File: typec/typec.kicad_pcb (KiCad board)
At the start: 2 copper layers, 76 parts, among them U1 TPD6E05U06-USON, U2 TPD4E05U06-USON, U3 TPS62081-WSON, U4 TPD4E05U06-USON, U5 TPS74801-VSON, U6 TUSB212-X2QFN, U7 USB_HUB, Y1 24 MHz

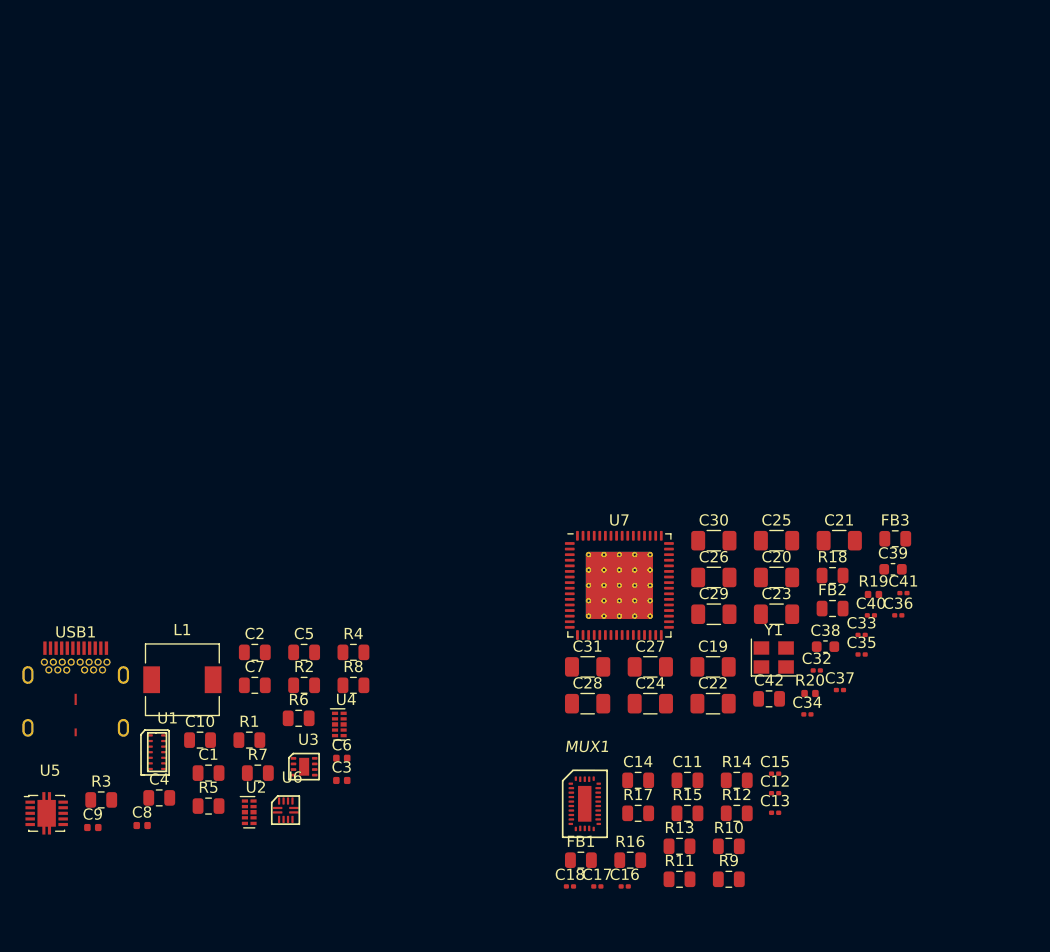
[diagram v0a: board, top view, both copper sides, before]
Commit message: Last minute changes
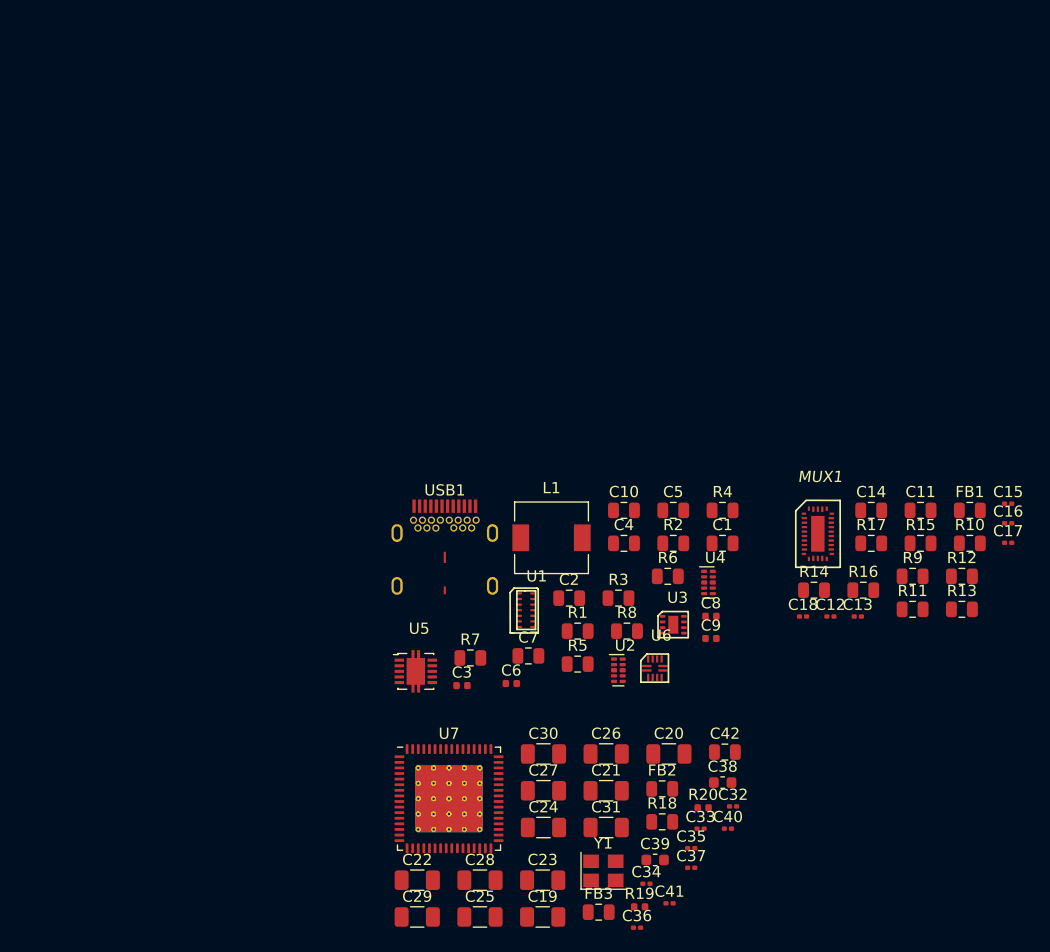
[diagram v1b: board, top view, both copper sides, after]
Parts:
- moved C9 57.8 mm to (154.3, 87.4)
- moved C8 54.2 mm to (154.3, 85.4)
- moved C1 50.4 mm to (155.3, 78.9)
- moved R3 49.7 mm to (146.0, 83.8)
- moved C17 47.9 mm to (180.9, 78.8)
- moved C4 47.4 mm to (146.5, 78.9)
- moved C16 47.2 mm to (180.9, 77.1)
- moved FB1 46.8 mm to (177.5, 75.9)
- moved C10 43.1 mm to (146.5, 75.9)
- moved C25 42.9 mm to (133.6, 112.3)
- moved FB3 42.7 mm to (144.3, 111.8)
- moved C29 37.9 mm to (128.0, 112.3)
- moved C36 36.4 mm to (147.7, 113.2)
- moved L1 35.4 mm to (140.0, 78.4)
- moved C5 35.4 mm to (150.9, 75.9)
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
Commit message: updated
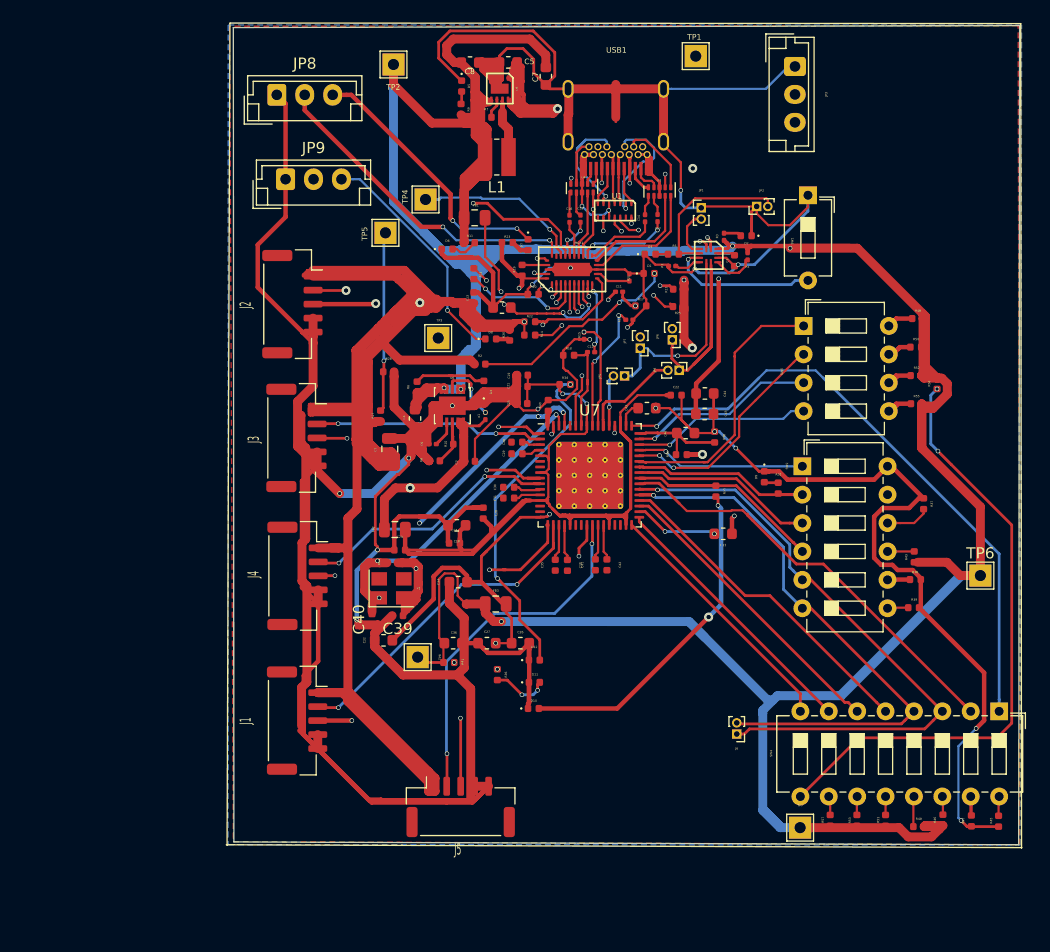
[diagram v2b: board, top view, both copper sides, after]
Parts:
- removed C37: 0.1uF/10v, Capacitor_SMD:C_0201_0603Metric
- removed C9: 0.1uF/10v, Capacitor_SMD:C_0402_1005Metric
- added C43: 1uF/10v, Capacitor_SMD:C_0603_1608Metric, F.Cu at (148.6, 66.8)
- added C44: 1uf/10v, Capacitor_SMD:C_0603_1608Metric, F.Cu at (153.8, 65.4)
- added C45: 1uf/10v, Capacitor_SMD:C_0603_1608Metric, F.Cu at (153.7, 67.3)
- added C46: 10 uF/10v, Capacitor_SMD:C_0603_1608Metric, F.Cu at (152.0, 69.0)
- added D1: LED, LED_SMD:LED_0402_1005Metric, F.Cu at (148.8, 54.7)
- added D10: LED, LED_SMD:LED_0402_1005Metric, F.Cu at (138.4, 93.6)
- added D11: LED, LED_SMD:LED_0402_1005Metric, F.Cu at (138.5, 91.3)
- added D12: LED, LED_SMD:LED_0402_1005Metric, F.Cu at (138.5, 89.3)
- added D2: LED, LED_SMD:LED_0402_1005Metric, F.Cu at (157.5, 51.3)
- added D3: LED, LED_SMD:LED_0402_1005Metric, F.Cu at (148.9, 53.0)
- added D4: LED, LED_SMD:LED_0402_1005Metric, F.Cu at (134.0, 64.8)
- added D5: LED, LED_SMD:LED_0402_1005Metric, F.Cu at (132.0, 38.0)
- added D6: LED, LED_SMD:LED_0402_1005Metric, F.Cu at (130.7, 52.5)
- added D7: LED, LED_SMD:LED_0402_1005Metric, F.Cu at (137.9, 52.1)
- added D8: LED, LED_SMD:LED_0402_1005Metric, F.Cu at (134.6, 60.6)
- added D9: LED, LED_SMD:LED_0402_1005Metric, F.Cu at (159.1, 72.9)
- added J1: Conn_01x05_Female, Connector_JST:JST_GH_SM05B-GHS-TB_1x05-1MP_P1.25mm_Horizontal, F.Cu at (117.3, 94.7)
- added J2: Conn_01x05_Female, Connector_JST:JST_GH_SM05B-GHS-TB_1x05-1MP_P1.25mm_Horizontal, F.Cu at (116.9, 57.5)
- added J3: Conn_01x05_Female, Connector_JST:JST_GH_SM05B-GHS-TB_1x05-1MP_P1.25mm_Horizontal, F.Cu at (117.2, 69.4)
- added J4: Conn_01x05_Female, Connector_JST:JST_GH_SM05B-GHS-TB_1x05-1MP_P1.25mm_Horizontal, F.Cu at (117.3, 81.8)
- added J5: Conn_01x05_Female, Connector_JST:JST_GH_SM05B-GHS-TB_1x05-1MP_P1.25mm_Horizontal, F.Cu at (131.9, 102.4)
- added J6: Conn_01x02_Female, Connector_PinHeader_1.00mm:PinHeader_1x02_P1.00mm_Vertical, F.Cu at (156.6, 95.9)
- added JP1: Jumper_NO_Small, Connector_PinHeader_1.00mm:PinHeader_1x02_P1.00mm_Vertical, F.Cu at (153.4, 48.8)
- added JP2: Jumper_NO_Small, Connector_PinHeader_1.00mm:PinHeader_1x02_P1.00mm_Vertical, F.Cu at (158.4, 48.7)
- added JP3: Jumper_3_Open, Connector_JST:JST_EH_B3B-EH-A_1x03_P2.50mm_Vertical, F.Cu at (161.8, 36.2)
- added JP4: Jumper_2_Open, Connector_PinHeader_1.00mm:PinHeader_1x02_P1.00mm_Vertical, F.Cu at (151.5, 63.4)
- added JP5: Jumper_2_Open, Connector_PinHeader_1.00mm:PinHeader_1x02_P1.00mm_Vertical, F.Cu at (146.6, 63.9)
- added JP6: Jumper_2_Open, Connector_PinHeader_1.00mm:PinHeader_1x02_P1.00mm_Vertical, F.Cu at (150.9, 60.7)
- added JP7: Jumper_2_Open, Connector_PinHeader_1.00mm:PinHeader_1x02_P1.00mm_Vertical, F.Cu at (148.0, 61.4)
- added JP8: Jumper_3_Open, Connector_JST:JST_EH_B3B-EH-A_1x03_P2.50mm_Vertical, F.Cu at (115.5, 38.7)
- added JP9: Jumper_3_Open, Connector_JST:JST_EH_B3B-EH-A_1x03_P2.50mm_Vertical, F.Cu at (116.3, 46.3)
- added R21: 0 E, Resistor_SMD:R_0201_0603Metric, F.Cu at (147.0, 55.1)
- added R22: 200 K, Resistor_SMD:R_0402_1005Metric, F.Cu at (138.1, 59.0)
- added R23: 500 E, Resistor_SMD:R_0402_1005Metric, F.Cu at (136.1, 51.9)
- added R25: 200 K, Resistor_SMD:R_0402_1005Metric, F.Cu at (151.4, 57.7)
- added R26: 500 E, Resistor_SMD:R_0402_1005Metric, F.Cu at (136.3, 60.2)
- added R27: NC / 10 K, Resistor_SMD:R_0402_1005Metric, F.Cu at (124.8, 67.5)
- added R28: NC/ 10 K, Resistor_SMD:R_0402_1005Metric, F.Cu at (125.5, 63.5)
- added R31: 330 E, Resistor_SMD:R_0402_1005Metric, F.Cu at (160.3, 73.9)
- added R34: 330 E, Resistor_SMD:R_0402_1005Metric, F.Cu at (141.2, 64.6)
- added R35: 330 E, Resistor_SMD:R_0402_1005Metric, F.Cu at (154.7, 74.2)
- added R36: 330 E, Resistor_SMD:R_0402_1005Metric, F.Cu at (135.2, 90.6)
- added R37: 1 K, Resistor_SMD:R_0402_1005Metric, F.Cu at (173.3, 75.3)
- added R38: 1 K, Resistor_SMD:R_0402_1005Metric, F.Cu at (172.6, 82.1)
- added R39: 1 K, Resistor_SMD:R_0402_1005Metric, F.Cu at (172.4, 84.6)
- added R40: 9.53 K, Resistor_SMD:R_0402_1005Metric, F.Cu at (139.8, 66.5)
- added R41: 1 K, Resistor_SMD:R_0402_1005Metric, F.Cu at (130.9, 89.5)
- added R43: 1 K, Resistor_SMD:R_0402_1005Metric, F.Cu at (172.5, 80.1)
- added R44: 1 M, Resistor_SMD:R_0402_1005Metric, F.Cu at (125.8, 80.6)
- added R45: 1 K, Resistor_SMD:R_0402_1005Metric, F.Cu at (180.0, 103.7)
- added R46: 1 K, Resistor_SMD:R_0402_1005Metric, F.Cu at (175.1, 103.6)
- added R47: 1 K, Resistor_SMD:R_0402_1005Metric, F.Cu at (177.6, 103.7)
- added R48: 10 K, Resistor_SMD:R_0402_1005Metric, F.Cu at (172.8, 58.7)
- added R49: 1 K, Resistor_SMD:R_0402_1005Metric, F.Cu at (172.9, 104.2)
- added R50: 10 K, Resistor_SMD:R_0402_1005Metric, F.Cu at (172.6, 61.3)
- added R51: 4.7 K, Resistor_SMD:R_0402_1005Metric, F.Cu at (169.9, 103.6)
- added R52: 10 K, Resistor_SMD:R_0402_1005Metric, F.Cu at (172.7, 63.8)
- added R53: 4.7 K, Resistor_SMD:R_0402_1005Metric, F.Cu at (167.4, 103.6)
- added R54: 90.9 K, Resistor_SMD:R_0402_1005Metric, F.Cu at (151.7, 70.9)
- added R55: 10 K, Resistor_SMD:R_0402_1005Metric, F.Cu at (172.7, 66.4)
- added R56: 10 K, Resistor_SMD:R_0402_1005Metric, F.Cu at (154.6, 69.3)
- added R57: 4.7 K, Resistor_SMD:R_0402_1005Metric, F.Cu at (165.0, 103.6)
- added R58: 4.7 K, Resistor_SMD:R_0402_1005Metric, F.Cu at (174.5, 64.6)
- added SW1: SW_Push_Dual_x2, Button_Switch_THT:SW_DIP_SPSTx01_Slide_6.7x4.1mm_W7.62mm_P2.54mm_LowProfile, F.Cu at (163.0, 47.7)
- added SW2: SW_DIP_x06, Button_Switch_THT:SW_DIP_SPSTx06_Slide_6.7x16.8mm_W7.62mm_P2.54mm_LowProfile, F.Cu at (162.5, 72.0)
- added SW4: SW_DIP_x08, Button_Switch_THT:SW_DIP_SPSTx08_Slide_6.7x21.88mm_W7.62mm_P2.54mm_LowProfile, F.Cu at (180.1, 93.9)
- added SW5: SW_DIP_x04, Button_Switch_THT:SW_DIP_SPSTx04_Slide_6.7x11.72mm_W7.62mm_P2.54mm_LowProfile, F.Cu at (162.6, 59.4)
- added TP1: TestPoint, TestPoint:TestPoint_THTPad_2.0x2.0mm_Drill1.0mm, F.Cu at (152.9, 35.3)
- added TP2: TestPoint, TestPoint:TestPoint_THTPad_2.0x2.0mm_Drill1.0mm, F.Cu at (125.9, 36.0)
- added TP3: TestPoint, TestPoint:TestPoint_THTPad_2.0x2.0mm_Drill1.0mm, F.Cu at (129.9, 60.5)
- added TP4: TestPoint, TestPoint:TestPoint_THTPad_2.0x2.0mm_Drill1.0mm, F.Cu at (128.8, 48.1)
- added TP5: TestPoint, TestPoint:TestPoint_THTPad_2.0x2.0mm_Drill1.0mm, F.Cu at (125.2, 51.1)
- added TP6: TestPoint, TestPoint:TestPoint_THTPad_2.0x2.0mm_Drill1.0mm, F.Cu at (178.4, 81.7)
- added TP7: TestPoint, TestPoint:TestPoint_THTPad_2.0x2.0mm_Drill1.0mm, F.Cu at (162.3, 104.3)
- added TP8: TestPoint, TestPoint:TestPoint_THTPad_2.0x2.0mm_Drill1.0mm, F.Cu at (128.1, 89.0)
- added e1: 105 K, Resistor_SMD:R_0201_0603Metric, F.Cu at (134.1, 67.5)
- C10: value 10uf/10v -> 0.1uf/10v; footprint Capacitor_SMD:C_0805_2012Metric -> Capacitor_SMD:C_0603_1608Metric
- C11: value 0.1uf/10v -> 0.47uf/10v; footprint Capacitor_SMD:C_0805_2012Metric -> Capacitor_SMD:C_0201_0603Metric
- C13: value 0.47uf/10v -> 4.7uf/10v; footprint Capacitor_SMD:C_0201_0603Metric -> Capacitor_SMD:C_0402_1005Metric
- C14: value 47uf/10v -> 0.4uf/10v; footprint Capacitor_SMD:C_0805_2012Metric -> Capacitor_SMD:C_0201_0603Metric
- C15: value 0.4uf/10v -> 0.47uf/10v
- C16: value 0.47uf/10v -> 0.4uf/10v
- C18: value 0.4uf/10v -> 10uF/10v; footprint Capacitor_SMD:C_0201_0603Metric -> Capacitor_SMD:C_0603_1608Metric
- C19, C20, C21, C22, C23, C24, C25, C28, C29, C30: footprint Capacitor_SMD:C_1206_3216Metric -> Capacitor_SMD:C_0402_1005Metric
- C2: value 10uf/10v -> 0.1uF/10v; footprint Capacitor_SMD:C_0805_2012Metric -> Capacitor_SMD:C_0402_1005Metric
- C26: value 10uF/10v -> 0.1uF/10v; footprint Capacitor_SMD:C_1206_3216Metric -> Capacitor_SMD:C_0603_1608Metric
- C27: footprint Capacitor_SMD:C_1206_3216Metric -> Capacitor_SMD:C_0603_1608Metric
- C3: value 1uf/10v -> 10uf/10v
- C31: value 10uF/10v -> 0.1uF/10v; footprint Capacitor_SMD:C_1206_3216Metric -> Capacitor_SMD:C_0402_1005Metric
- C32, C33: footprint Capacitor_SMD:C_0201_0603Metric -> Capacitor_SMD:C_0603_1608Metric
- C34: value 0.1uF/10v -> 10uF/10v; footprint Capacitor_SMD:C_0201_0603Metric -> Capacitor_SMD:C_0603_1608Metric
- C35, C41: footprint Capacitor_SMD:C_0201_0603Metric -> Capacitor_SMD:C_0402_1005Metric
- C36: value 0.1uF/10v -> 1uf/10v; footprint Capacitor_SMD:C_0201_0603Metric -> Capacitor_SMD:C_0603_1608Metric
- C38: value 18pF/10v -> 0.1uF/10v; footprint Capacitor_SMD:C_0603_1608Metric -> Capacitor_SMD:C_0402_1005Metric
- C39: footprint Capacitor_SMD:C_0603_1608Metric -> Capacitor_SMD:C_0402_1005Metric
- C4: value 10 uF/10V -> 1uf/10v; footprint Capacitor_SMD:C_0805_2012Metric -> Capacitor_SMD:C_0603_1608Metric
- C40: value 0.1uF/10v -> 18pF/10v; footprint Capacitor_SMD:C_0201_0603Metric -> Capacitor_SMD:C_0402_1005Metric
- C42: value 1uF/10v -> 0.1uF/10v; footprint Capacitor_SMD:C_0805_2012Metric -> Capacitor_SMD:C_0402_1005Metric
- C5: value 22uf/6.3v -> 10 uF/10V; footprint Capacitor_SMD:C_0805_2012Metric -> Capacitor_SMD:C_0603_1608Metric
- C6: value 560pf/10v -> 590pf/10v; footprint Capacitor_SMD:C_0402_1005Metric -> Capacitor_SMD:C_0201_0603Metric
- C7: value 10uf/10v -> 22uf/6.3v; footprint Capacitor_SMD:C_0805_2012Metric -> Capacitor_SMD:C_0603_1608Metric
- C8: value 0.1uF/10v -> 10uf/10v; footprint Capacitor_SMD:C_0402_1005Metric -> Capacitor_SMD:C_0603_1608Metric
- L1: footprint Inductor_SMD:L_6.3x6.3_H3 -> Inductor_SMD:L_Wuerth_MAPI-3015
- R1: value 105 K -> 1.6K; footprint Resistor_SMD:R_0805_2012Metric -> Resistor_SMD:R_0201_0603Metric
- R10: value 10 K -> 1.9K; footprint Resistor_SMD:R_0805_2012Metric -> Resistor_SMD:R_0402_1005Metric
- R11: value 900 K -> 330 E; footprint Resistor_SMD:R_0805_2012Metric -> Resistor_SMD:R_0402_1005Metric
- R12, R15: footprint Resistor_SMD:R_0805_2012Metric -> Resistor_SMD:R_0201_0603Metric
- R13: value 4.7K -> 10 K; footprint Resistor_SMD:R_0805_2012Metric -> Resistor_SMD:R_0402_1005Metric
- R14: value 100K -> 900 K; footprint Resistor_SMD:R_0805_2012Metric -> Resistor_SMD:R_0402_1005Metric
- R16: value 0 E -> 4.7K; footprint Resistor_SMD:R_0805_2012Metric -> Resistor_SMD:R_0402_1005Metric
- R17: value 0 E -> 100K; footprint Resistor_SMD:R_0805_2012Metric -> Resistor_SMD:R_0402_1005Metric
- R18: value 1 M -> 100K; footprint Resistor_SMD:R_0805_2012Metric -> Resistor_SMD:R_0402_1005Metric
- R19: value 4.7K -> 200 K
- R2: value 178K -> 330 E; footprint Resistor_SMD:R_0805_2012Metric -> Resistor_SMD:R_0402_1005Metric
- R20: value 4.7K -> 0 E
- R3: value 5 K -> 330 E; footprint Resistor_SMD:R_0805_2012Metric -> Resistor_SMD:R_0201_0603Metric
- R4: value 1.9K -> 43K; footprint Resistor_SMD:R_0805_2012Metric -> Resistor_SMD:R_0201_0603Metric
- R5: value 1.6K -> 100 E; footprint Resistor_SMD:R_0805_2012Metric -> Resistor_SMD:R_0402_1005Metric
- R6: value 43K -> 330 E; footprint Resistor_SMD:R_0805_2012Metric -> Resistor_SMD:R_0402_1005Metric
- R7: value 0 E -> 178K; footprint Resistor_SMD:R_0805_2012Metric -> Resistor_SMD:R_0402_1005Metric
- R8: value 0 E -> 5 K; footprint Resistor_SMD:R_0805_2012Metric -> Resistor_SMD:R_0402_1005Metric
- R9: value 100K -> 330 E; footprint Resistor_SMD:R_0805_2012Metric -> Resistor_SMD:R_0402_1005Metric
- U2: value TPD4E05U06-USON -> TUSB212-X2QFN; footprint TPD4E05U06-USON:TPD4E05U06-USON -> TUSB212-X2QFN:TUSB212-X2QFN
- U3: value TPS62081-WSON -> TPD4E05U06-USON; footprint TPS62081-WSON:TPS62081-WSON -> TPD4E05U06-USON:TPD4E05U06-USON
- U5: value TPS74801-VSON -> TPS62082-WSON; footprint TPS74801-VSON:TPS74801-VSON -> TPS62081-WSON:TPS62082-WSON
- U6: value TUSB212-X2QFN -> TPS74801-VSON; footprint TUSB212-X2QFN:TUSB212-X2QFN -> TPS74801-VSON:TPS74801-VSON
- moved R9 58.1 mm to (132.0, 40.0), turned to 90 degrees
- moved R19 57.9 mm to (137.4, 54.4), turned to 270 degrees
- moved C8 54.0 mm to (132.8, 35.8)
- moved USB1 53.6 mm to (145.8, 34.7), turned to 180 degrees
- moved U5 52.8 mm to (135.0, 37.9), turned to 270 degrees
- moved C7 51.9 mm to (139.5, 37.1), turned to 270 degrees
- moved R11 51.5 mm to (132.7, 52.0)
- moved FB1 51.4 mm to (133.2, 49.7)
- moved C22 49.2 mm to (151.2, 65.6), turned to 180 degrees
- moved C19 48.5 mm to (137.4, 63.8)
- moved R20 48.4 mm to (138.4, 56.6)
- moved R7 48.4 mm to (134.2, 40.7), turned to 180 degrees
- moved C16 47.8 mm to (141.7, 49.8), turned to 90 degrees
- moved R10 46.6 mm to (131.7, 70.0), turned to 180 degrees
- moved C25 46.1 mm to (137.4, 66.3)
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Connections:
- C1 pad 1: VOUT(1.1V) -> VBUS
- C1 pad 2: USB3_RX0N -> GND
- C10 pad 1: VBUS -> Net-(C10-Pad1)
- C10 pad 2: USB3_RX0N -> GND
- C12 pad 2: USB3_RX0N -> USB3_RX0P
- C13 pad 1: Net-(C13-Pad1) -> GND
- C13 pad 2: USB3_RX0N -> VBUS
- C14 pad 1: USB3_RX0N -> CTX1N0
- C14 pad 2: VBUS -> Net-(C14-Pad2)
- C15 pad 1: CTX1N -> Net-(C15-Pad1)
- C15 pad 2: Net-(C15-Pad2) -> CTX2P0
- C16 pad 2: CTX2P -> CTX2N0
- C17 pad 2: CTX2N -> CTX1P0
- C18 pad 2: CTX1P -> GND
- C19 pad 1: USB3_RX0N -> GND
- C19 pad 2: Net-(C19-Pad2) -> Net-(C18-Pad1)
- C2 pad 1: VBUS -> Net-(C2-Pad1)
- C2 pad 2: USB3_RX0N -> GND
- C20 pad 1: USB3_RX0N -> GND
- C20 pad 2: Net-(C19-Pad2) -> Net-(C18-Pad1)
- C21 pad 1: USB3_RX0N -> GND
- C21 pad 2: Net-(C19-Pad2) -> Net-(C18-Pad1)
- C22 pad 1: USB3_RX0N -> GND
- C22 pad 2: Net-(C19-Pad2) -> Net-(C18-Pad1)
- C23 pad 1: USB3_RX0N -> GND
- C23 pad 2: Net-(C19-Pad2) -> Net-(C18-Pad1)
- C24 pad 1: USB3_RX0N -> GND
- C24 pad 2: Net-(C19-Pad2) -> Net-(C18-Pad1)
- C25 pad 1: USB3_RX0N -> GND
- C25 pad 2: Net-(C19-Pad2) -> Net-(C18-Pad1)
- C26 pad 1: Net-(C19-Pad2) -> GND
- C26 pad 2: USB3_RX0N -> Net-(C26-Pad2)
- C27 pad 1: USB3_RX0N -> GND
- C27 pad 2: Net-(C27-Pad2) -> Net-(C26-Pad2)
- C28 pad 1: USB3_RX0N -> (no net)
- C28 pad 2: Net-(C27-Pad2) -> Net-(C28-Pad2)
- C29 pad 1: USB3_RX0N -> Net-(C29-Pad1)
- C29 pad 2: Net-(C27-Pad2) -> (no net)
- C3 pad 1: Net-(C3-Pad1) -> VOUT(1.1V)
- C3 pad 2: USB3_RX0N -> GND
- C30 pad 1: USB3_RX0N -> (no net)
- C30 pad 2: Net-(C27-Pad2) -> Net-(C30-Pad2)
- C31 pad 1: Net-(C27-Pad2) -> Net-(C31-Pad1)
- C31 pad 2: USB3_RX0N -> (no net)
- C32 pad 1: Tx1+ -> GND
- C32 pad 2: Net-(C32-Pad2) -> Net-(C26-Pad2)
- C33 pad 1: Net-(C33-Pad1) -> GND
- C33 pad 2: Tx1- -> Net-(C26-Pad2)
- C34 pad 1: Tx2+ -> Net-(C26-Pad2)
- C34 pad 2: Net-(C34-Pad2) -> GND
- C35 pad 1: Net-(C35-Pad1) -> (no net)
- C35 pad 2: Tx2- -> Net-(C35-Pad2)
- C36 pad 1: Tx3+ -> VOUT(3.3V)
- C36 pad 2: Net-(C36-Pad2) -> GND
- C38 pad 2: USB3_RX0N -> (no net)
- C39 pad 1: USB3_RX0N -> Net-(C39-Pad1)
- C39 pad 2: Net-(C39-Pad2) -> GND
- C4 pad 1: VBUS -> VOUT(3.3V)
- C4 pad 2: USB3_RX0N -> GND
- C40 pad 1: Tx4+ -> GND
- C41 pad 1: Net-(C41-Pad1) -> (no net)
- C41 pad 2: Tx4- -> Net-(C41-Pad2)
- C42 pad 2: USB3_RX0N -> (no net)
- C5 pad 1: VOUT(3.3V) -> VBUS
- C5 pad 2: USB3_RX0N -> GND
- C6 pad 2: USB3_RX0N -> GND
- C7 pad 2: USB3_RX0N -> GND
- C8 pad 1: USB3_RX0N -> VOUT(3.3V)
- C8 pad 2: Net-(C8-Pad2) -> GND
- FB1 pad 2: Net-(C11-Pad1) -> Net-(C10-Pad1)
- FB2 pad 2: Net-(C19-Pad2) -> Net-(C18-Pad1)
- FB3 pad 2: Net-(C27-Pad2) -> Net-(C26-Pad2)
- MUX1 pad 1: CC2 -> CC20
- MUX1 pad 10: Net-(C13-Pad1) -> Net-(C12-Pad1)
- MUX1 pad 11: Net-(MUX1-Pad11) -> DIR
- MUX1 pad 13: USB3_RX0N -> GND
- MUX1 pad 14: CRX1N -> CRX1N0
- MUX1 pad 15: CRX1P -> CRX1P0
- MUX1 pad 16: Net-(C15-Pad2) -> Net-(C14-Pad2)
- MUX1 pad 17: Net-(C18-Pad1) -> Net-(C17-Pad1)
- MUX1 pad 18: CRX2N -> CRX2N0
- MUX1 pad 19: CRX2P -> CRX2P0
- MUX1 pad 2: CC1 -> CC10
- MUX1 pad 20: Net-(C17-Pad1) -> Net-(C16-Pad1)
- MUX1 pad 21: Net-(C16-Pad1) -> Net-(C15-Pad1)
- MUX1 pad 22: Net-(MUX1-Pad22) -> ADDR
- MUX1 pad 23: Net-(MUX1-Pad23) -> INT_NOUT3
- MUX1 pad 24: Net-(MUX1-Pad24) -> (no net)
- MUX1 pad 25: Net-(MUX1-Pad25) -> SDAOUT1
- MUX1 pad 26: Net-(MUX1-Pad26) -> SCLOUT2
- MUX1 pad 28: USB3_RX0N -> GND
- MUX1 pad 31: (no net) -> GND
- MUX1 pad 8: Net-(C11-Pad1) -> Net-(C10-Pad1)
- MUX1 pad 9: Net-(C12-Pad1) -> Net-(C11-Pad1)
- R1 pad 1: VOUT(1.1V) -> Net-(R1-Pad1)
- R1 pad 2: Net-(R1-Pad2) -> GND
- R10 pad 1: Net-(MUX1-Pad3) -> VOUT(1.1V)
- R10 pad 2: VBUS -> Net-(R10-Pad2)
- R11 pad 1: Net-(MUX1-Pad5) -> VOUT(3.3V)
- R11 pad 2: VBUS -> Net-(D6-Pad2)
- R12 pad 1: USB3_RX0N -> USB3_TX0N
- R12 pad 2: USB3_TX0P -> GND
- R13 pad 1: Net-(MUX1-Pad4) -> Net-(MUX1-Pad3)
- R13 pad 2: USB3_RX0N -> VBUS
- R14 pad 1: USB3_RX0N -> Net-(MUX1-Pad5)
- R14 pad 2: USB3_RX0N -> VBUS
- R15 pad 1: USB3_RX0N -> GND
- R15 pad 2: USB3_RX0N -> USB3_TX0P
- R16 pad 1: USB3_RX0N -> Net-(JP3-Pad2)
- R16 pad 2: Net-(MUX1-Pad29) -> Net-(MUX1-Pad4)
- R17 pad 1: Net-(MUX1-Pad12) -> USB3_RX0N
- R17 pad 2: USB3_RX0N -> GND
- R18 pad 1: Net-(C38-Pad1) -> USB3_RX0P
- R18 pad 2: Net-(C39-Pad2) -> GND
- R19 pad 1: USB3_RX0N -> Net-(MUX1-Pad27)
- R19 pad 2: Net-(R19-Pad2) -> VBUS
- R2 pad 1: Net-(R2-Pad1) -> VBUS
- R2 pad 2: VOUT(3.3V) -> Net-(D1-Pad2)
- R20 pad 1: USB3_RX0N -> GND
- R20 pad 2: Net-(R20-Pad2) -> Net-(MUX1-Pad29)
- R3 pad 1: USB3_RX0N -> VOUT(3.3V)
- R3 pad 2: Net-(R3-Pad2) -> Net-(D2-Pad2)
- R4 pad 1: VOUT(1.1V) -> VOUT(3.3V)
- R4 pad 2: Net-(R3-Pad2) -> Net-(R4-Pad2)
- R5 pad 1: Net-(R5-Pad1) -> SCL
- R5 pad 2: USB3_RX0N -> Net-(D3-Pad2)
- R6 pad 2: Net-(R6-Pad2) -> Net-(D4-Pad2)
- R7 pad 1: CC1 -> Net-(R7-Pad1)
- R7 pad 2: Net-(R7-Pad2) -> VOUT(3.3V)
- R8 pad 1: CC2 -> GND
- R8 pad 2: Net-(R8-Pad2) -> Net-(R10-Pad2)
- R9 pad 1: USB3_TX0N -> VOUT(3.3V)
- R9 pad 2: USB3_RX0N -> Net-(D5-Pad2)
- U1 pad 10: USB3_RX0N -> GND
- U1 pad 13: CC2 -> (no net)
- U1 pad 14: CC1 -> CC10
- U1 pad 2: CC2 -> CSBU2
- U1 pad 3: USB2_N0 -> USB2_N
- U1 pad 4: USB2_P0 -> USB2_P
- U1 pad 5: USB3_RX0N -> GND
- U1 pad 6: CSBU2 -> CC2
- U1 pad 8: CSBU1 -> (no net)
- U1 pad 9: CSBU2 -> CC20
- U2 pad 1: CTX1N -> USB2_N0
- U2 pad 10: CTX1N -> GND
- U2 pad 2: CTX1P -> USB2_P0
- U2 pad 3: USB3_RX0N -> Net-(JP1-Pad2)
- U2 pad 4: CRX1N -> SCL
- U2 pad 5: CRX1P -> Net-(SW1-Pad2)
- U2 pad 6: CRX1P -> Net-(R1-Pad1)
- U2 pad 7: CRX1N -> USB2_P10
- U2 pad 8: USB3_RX0N -> USB2_N10
- U2 pad 9: CTX1P -> Net-(R4-Pad2)
- U3 pad 1: VBUS -> CRX1N
- U3 pad 2: USB3_RX0N -> CRX1P
- U3 pad 3: USB3_RX0N -> GND
- U3 pad 4: USB3_RX0N -> CTX1P
- U3 pad 5: VOUT(3.3V) -> CTX1N
- U3 pad 6: Net-(R2-Pad1) -> CTX1N0
- U3 pad 7: Net-(L1-Pad1) -> CTX1P0
- U3 pad 8: VBUS -> GND
- U3 pad 9: (no net) -> CRX1P0
- U4 pad 1: CTX2N -> CRX2N
- U4 pad 10: CTX2N -> CRX2N0
- U4 pad 2: CTX2P -> CRX2P
- U4 pad 3: USB3_RX0N -> GND
- U4 pad 4: CRX2N -> CTX2P
- U4 pad 5: CRX2P -> CTX2N
- U4 pad 6: CRX2P -> CTX2N0
- U4 pad 7: CRX2N -> CTX2P0
- U4 pad 8: USB3_RX0N -> GND
- U4 pad 9: CTX2P -> CRX2P0
- U5 pad 2: VBUS -> GND
- U5 pad 3: Net-(R1-Pad2) -> GND
- U5 pad 4: Net-(C3-Pad1) -> GND
- U5 pad 5: Net-(C3-Pad1) -> VOUT(3.3V)
- U5 pad 6: USB3_RX0N -> Net-(R7-Pad1)
- U5 pad 7: Net-(C6-Pad1) -> Net-(L1-Pad1)
- U5 pad 8: Net-(R3-Pad2) -> VBUS
- U5 pad 9: VOUT(1.1V) -> GND
- U6 pad 1: USB2_N0 -> VOUT(3.3V)
- U6 pad 10: Net-(C9-Pad2) -> VOUT(1.1V)
- U6 pad 11: Net-(C9-Pad1) -> GND
- U6 pad 2: USB2_P0 -> VOUT(3.3V)
- U6 pad 4: Net-(U6-Pad4) -> VOUT(3.3V)
- U6 pad 5: Net-(C8-Pad2) -> VOUT(3.3V)
- U6 pad 6: Net-(R5-Pad1) -> GND
- U6 pad 7: USB2_P0 -> Net-(C6-Pad1)
- U6 pad 8: USB2_N0 -> Net-(R10-Pad2)
- U6 pad 9: Net-(R6-Pad2) -> VOUT(1.1V)
- U7 pad 11: Net-(C34-Pad2) -> Net-(C30-Pad2)
- U7 pad 12: Net-(C35-Pad1) -> Net-(C31-Pad1)
- U7 pad 13: Net-(C19-Pad2) -> Net-(C18-Pad1)
- U7 pad 14: Rx2+ -> (no net)
- U7 pad 15: Rx2- -> (no net)
- U7 pad 16: Net-(C27-Pad2) -> Net-(C26-Pad2)
- U7 pad 19: Net-(C36-Pad2) -> Net-(C35-Pad2)
- U7 pad 20: Net-(C37-Pad1) -> Net-(C38-Pad1)
- U7 pad 21: Net-(C19-Pad2) -> Net-(C18-Pad1)
- U7 pad 22: Rx3+ -> (no net)
- U7 pad 23: Rx3- -> (no net)
- U7 pad 26: Net-(C40-Pad2) -> Net-(C41-Pad2)
- U7 pad 27: Net-(C41-Pad1) -> Net-(C42-Pad1)
- U7 pad 28: Net-(C19-Pad2) -> Net-(C18-Pad1)
- U7 pad 29: Rx4+ -> (no net)
- U7 pad 3: Net-(C32-Pad2) -> Net-(C28-Pad2)
- U7 pad 30: Rx4- -> (no net)
- U7 pad 31: Net-(C19-Pad2) -> Net-(C18-Pad1)
- U7 pad 32: Net-(U7-Pad32) -> PWRON4_BATEN4
- U7 pad 33: Net-(U7-Pad33) -> PWRON3_BATEN3
- U7 pad 34: Net-(C27-Pad2) -> Net-(C26-Pad2)
- U7 pad 35: Net-(U7-Pad35) -> PWRON2_BATEN2
- U7 pad 36: Net-(U7-Pad36) -> PWRON1_BATEN1
- U7 pad 37: Net-(U7-Pad37) -> SDA_SMBDAT
- U7 pad 38: Net-(U7-Pad38) -> SCL_SMBCLK
- U7 pad 39: Net-(U7-Pad39) -> SMBUSZ
- U7 pad 4: Net-(C33-Pad1) -> Net-(C29-Pad1)
- U7 pad 40: Net-(R19-Pad2) -> FULLPWRMGMTZ_SS_UP
- U7 pad 41: Net-(U7-Pad41) -> PWRCTL_POL_TDO
- U7 pad 42: Net-(R20-Pad2) -> GANGED_HS_UP
- U7 pad 43: Net-(U7-Pad43) -> OVERCUR4z
- U7 pad 44: Net-(U7-Pad44) -> OVERCUR3z
- U7 pad 45: Net-(U7-Pad45) -> AUTOENZ
- U7 pad 46: Net-(U7-Pad46) -> OVERCUR1z
- U7 pad 47: Net-(U7-Pad47) -> OVERCUR2z
- U7 pad 49: Net-(U7-Pad49) -> TEST_TRSTZ
- U7 pad 5: Net-(C19-Pad2) -> Net-(C18-Pad1)
- U7 pad 50: Net-(C42-Pad1) -> Net-(C43-Pad1)
- U7 pad 51: Net-(C19-Pad2) -> Net-(C18-Pad1)
- U7 pad 52: Net-(C27-Pad2) -> Net-(C26-Pad2)
- U7 pad 55: Net-(U7-Pad55) -> USB3_TX0P
- U7 pad 56: Net-(U7-Pad56) -> USB3_TX0N
- U7 pad 57: Net-(C19-Pad2) -> Net-(C18-Pad1)
- U7 pad 58: Net-(U7-Pad58) -> USB3_RX0P
- U7 pad 59: Net-(U7-Pad59) -> USB3_RX0N
- U7 pad 6: Rx1+ -> (no net)
- U7 pad 60: Net-(U7-Pad60) -> (no net)
- U7 pad 61: Net-(C38-Pad1) -> Net-(C39-Pad1)
- U7 pad 62: Net-(C39-Pad2) -> Net-(C40-Pad2)
- U7 pad 63: Net-(C27-Pad2) -> Net-(C26-Pad2)
- U7 pad 65: (no net) -> GND
- U7 pad 7: Rx1- -> (no net)
- U7 pad 8: Net-(C19-Pad2) -> Net-(C18-Pad1)
- USB1 pad 1: USB3_RX0N -> GND
- USB1 pad 12: USB3_RX0N -> GND
- USB1 pad 13: USB3_RX0N -> GND
- USB1 pad 17: Net-(R8-Pad2) -> CC2
- USB1 pad 18: USB2_P0 -> USB2_P
- USB1 pad 19: USB2_N0 -> USB2_N
- USB1 pad 24: USB3_RX0N -> GND
- USB1 pad 25: Net-(USB1-Pad25) -> GND
- USB1 pad 26: Net-(USB1-Pad26) -> GND
- USB1 pad 27: Net-(USB1-Pad27) -> GND
- USB1 pad 5: Net-(R7-Pad2) -> CC1
- USB1 pad 6: USB2_N0 -> USB2_N
- USB1 pad 7: USB2_P0 -> USB2_P
- Y1 pad 1: Net-(C39-Pad2) -> Net-(C40-Pad2)
- Y1 pad 2: Net-(C38-Pad1) -> Net-(C39-Pad1)
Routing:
- net GND: track 0.00 -> 789.0 mm, vias 0 -> 21
- net VBUS: track 0.00 -> 720.6 mm, vias 0 -> 10
- net VOUT(3.3V): track 0.00 -> 490.6 mm, vias 0 -> 6
- net Net-(C18-Pad1): track 0.00 -> 116.5 mm, vias 0 -> 2
- net Net-(R41-Pad2): track 0.00 -> 72.1 mm, vias 0 -> 1
- net Net-(C26-Pad2): track 0.00 -> 69.7 mm, vias 0 -> 7
- net Net-(R58-Pad1): track 0.00 -> 57.7 mm, vias 0 -> 2
- net TEST_TRSTZ: track 0.00 -> 56.9 mm, vias 0 -> 1
- net SCL_SMBCLK: track 0.00 -> 55.8 mm, vias 0 -> 1
- net SDA_SMBDAT: track 0.00 -> 52.6 mm, vias 0 -> 1
- net Net-(J2-Pad2): track 0.00 -> 48.4 mm, vias 0 -> 1
- net Net-(C39-Pad1): track 0.00 -> 46.3 mm, vias 0 -> 4
- net ADDR: track 0.00 -> 41.7 mm, vias 0 -> 2
- net SMBUSZ: track 0.00 -> 40.1 mm
- net Net-(J2-Pad3): track 0.00 -> 38.2 mm, vias 0 -> 1
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- added copper zone on B.Cu, net (none)
- added copper zone on F.Cu, net (none)
- added copper zone on In1.Cu, net (none)
- added copper zone on In2.Cu, net (none)
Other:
- board outline added: 70.3 x 73.3 mm
- copper layers 2 -> 4
